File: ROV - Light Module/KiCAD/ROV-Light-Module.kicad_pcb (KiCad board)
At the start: 2 copper layers, 73.7 x 23.4 mm, 57 parts, among them J1 AVR UPDI Header, J4 Conn_02x05_Odd_Even, J6 Main In, J7 Conn_02x05_Odd_Even, J8 Middle - Top, J9 Middle - Top, U1 AL8805W5, U2 ATtiny1614-Arduino, U3 AP63205WU, U6 MAX13487E

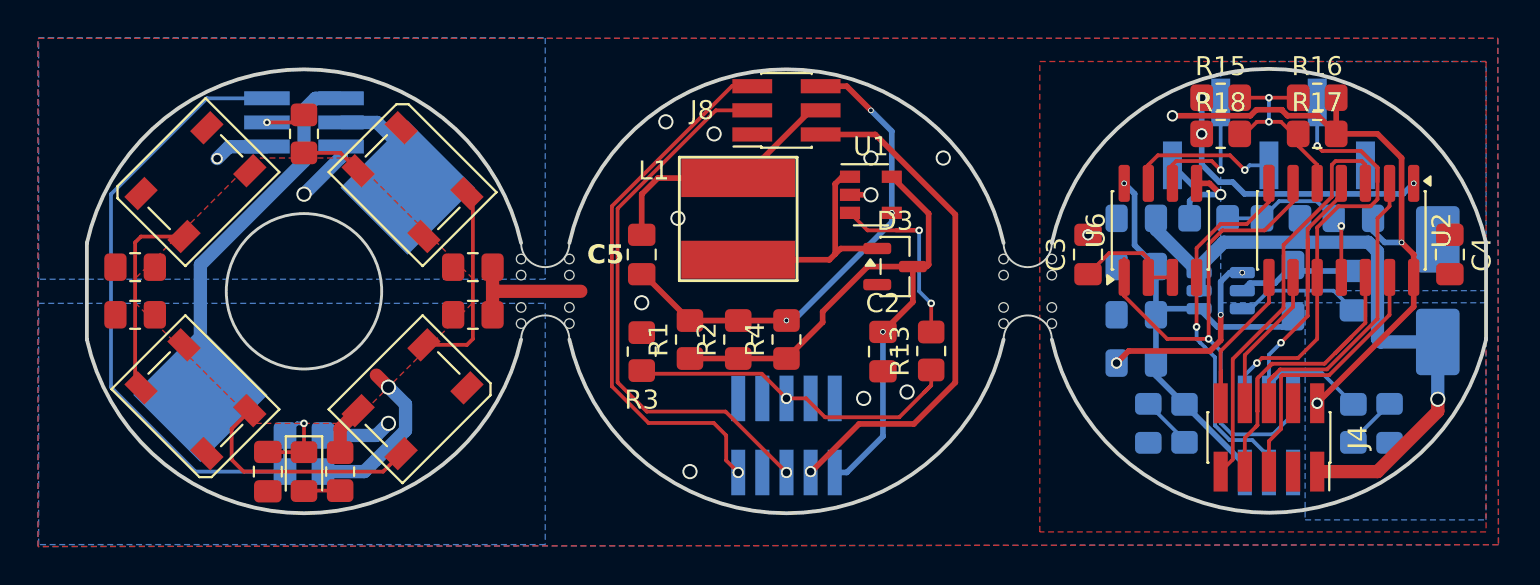
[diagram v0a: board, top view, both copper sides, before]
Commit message: clean up schematics
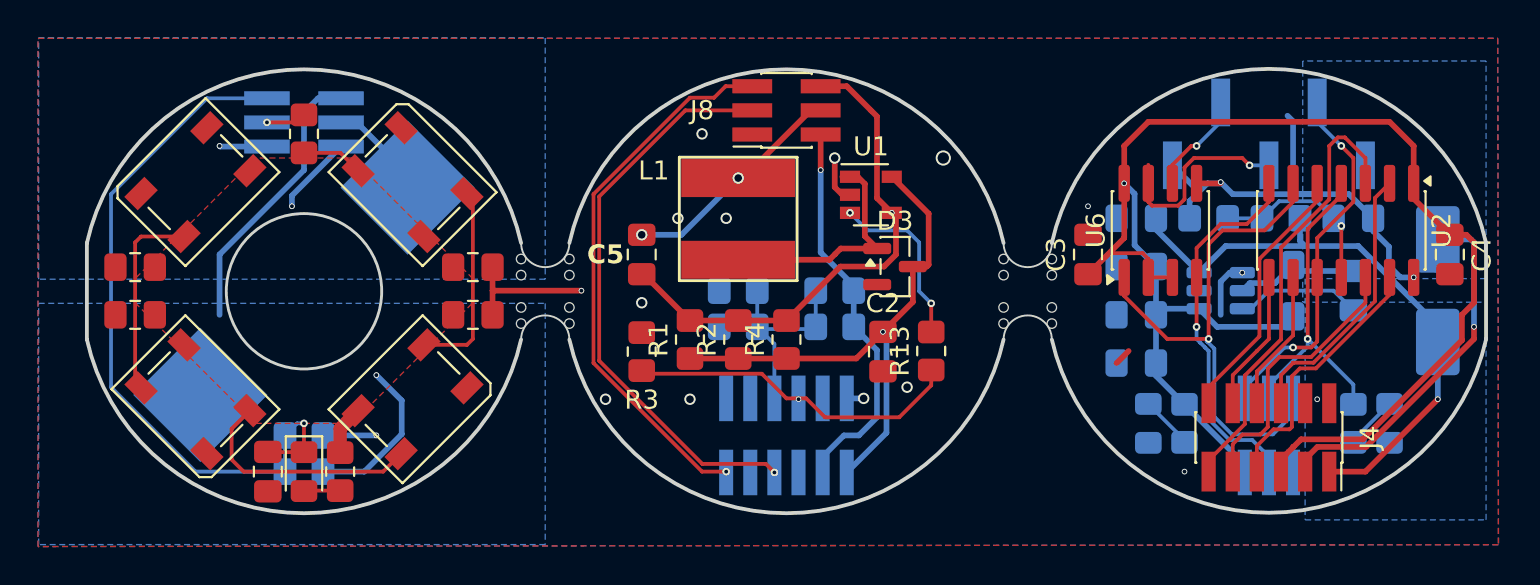
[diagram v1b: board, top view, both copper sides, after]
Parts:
- J4: value Conn_02x05_Odd_Even -> Conn_02x06_Odd_Even; footprint Connector_PinSocket_1.27mm:PinSocket_2x05_P1.27mm_Vertical_SMD -> Connector_PinSocket_1.27mm:PinSocket_2x06_P1.27mm_Vertical_SMD
- J7: value Conn_02x05_Odd_Even -> Conn_02x06_Odd_Even; footprint Connector_PinHeader_1.27mm:PinHeader_2x05_P1.27mm_Vertical_SMD -> Connector_PinHeader_1.27mm:PinHeader_2x06_P1.27mm_Vertical_SMD
- R15, R16, R17, R18: moved to B.Cu
- moved R16 32.1 mm to (162.6, 76.2), turned to 180 degrees
- moved R17 32.1 mm to (162.6, 78.1), turned to 180 degrees
- moved R18 22.7 mm to (167.6, 78.1), turned to 180 degrees
- moved R15 22.7 mm to (167.6, 76.2), turned to 180 degrees
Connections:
- J4 pad 3: +5V -> V_Supply
- J4 pad 5: /NeoPixle -> +5V
- J4 pad 7: /A9/D9 -> /NeoPixle
- J4 pad 9: /STATUS_LED -> /A9/D9
- J7 pad 5: /Neo_Mid -> unconnected-(J7-Pin_5-Pad5)
- J7 pad 7: unconnected-(J7-Pin_7-Pad7) -> /Neopixle_Mid
- J7 pad 8: unconnected-(J7-Pin_8-Pad8) -> /Function_Mid
- J7 pad 9: /STATUS -> unconnected-(J7-Pin_9-Pad9)
- J8 pad 3: /Neo_Mid -> /Neopixle_Mid
- R15 pad 1: +5V -> +5V_Mid
- R15 pad 2: /Function -> /Function_Mid
- R16 pad 1: /Function -> /Function_Mid
- R17 pad 1: /Function -> /Function_Mid
- R18 pad 1: +5V -> +5V_Mid
- R18 pad 2: /Function -> /Function_Mid
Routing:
- net +5V: track 49.6 -> 81.3 mm, vias 4 -> 1
- net /Neopixle_Mid: track 0.00 -> 30.2 mm, vias 0 -> 1
- net /Neo_Mid: track 29.2 -> 0.00 mm, vias 1 -> 0
- net V_Supply: track 0.00 -> 20.6 mm, vias 0 -> 1
- net GND: track 64.0 -> 45.6 mm, vias 20 -> 19
- net /Function_Mid: track 0.00 -> 11.1 mm
- net +5V_Mid: track 27.3 -> 20.7 mm
- net /Arduino Driver PCB/Builtin_LED: track 22.0 -> 16.6 mm
- net /LED+_U: track 19.5 -> 14.8 mm
- net /Arduino Driver PCB/UPDI: track 23.9 -> 19.6 mm
- net V_in_Mid: track 33.3 -> 29.5 mm
- net V_in: track 35.7 -> 32.4 mm
- net /A9/D9: track 17.9 -> 14.6 mm
- net /Arduino Driver PCB/Data_B: track 7.96 -> 10.6 mm
- net /STATUS_LED: track 21.5 -> 23.7 mm
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- removed copper zone on F.Cu, net +5V
